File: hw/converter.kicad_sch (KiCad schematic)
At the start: 16 parts, among them J301 1935776, J302 1935776, Q301 SW_L, Q302 SW_H

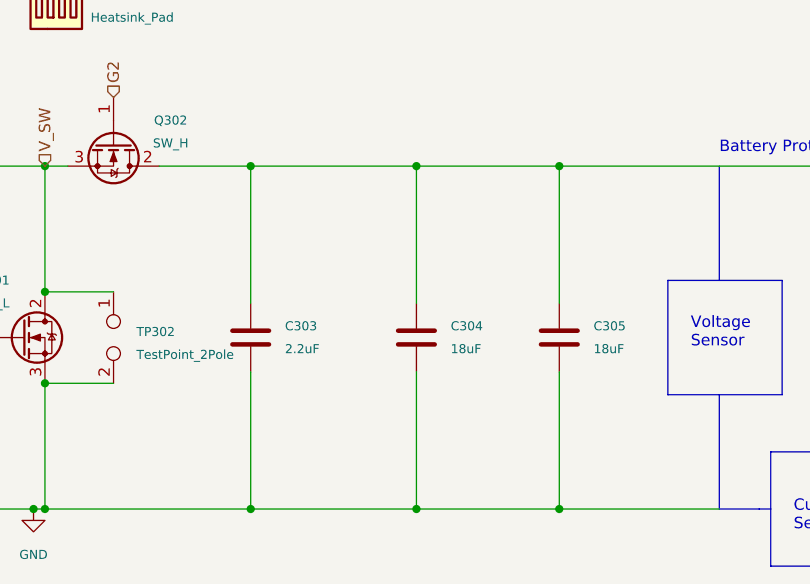
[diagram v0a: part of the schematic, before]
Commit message: hw changes
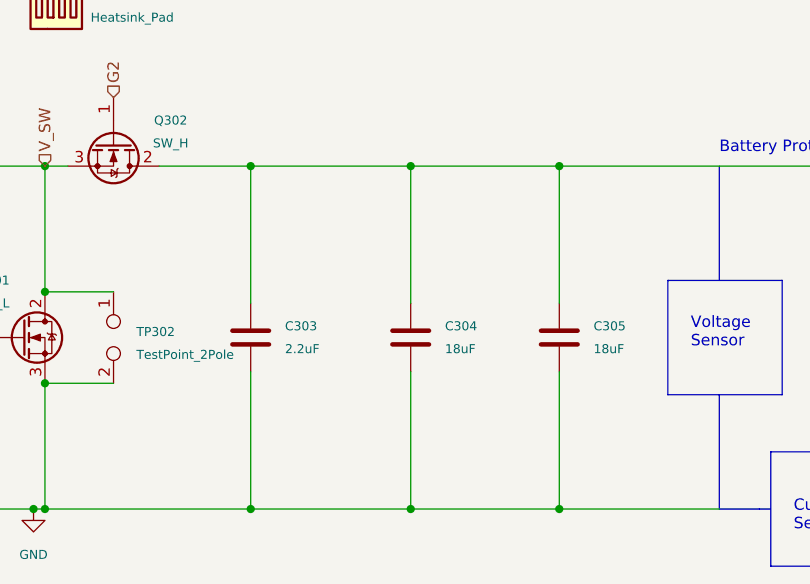
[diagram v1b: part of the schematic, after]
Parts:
- HS301: footprint mppt:WayinTop_HS -> footprints:WayinTop_HS
- J301, J302: footprint mppt:1935776 -> footprints:1935776
- L301: footprint mppt:B65878E1012D001 -> footprints:B65878E1012D001
- Q301, Q302: footprint mppt:EPC2307 -> footprints:EPC2307
- TP302, TP410: footprint mppt:SignalTP -> footprints:SignalTP
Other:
- moved on the sheet: C304
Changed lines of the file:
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@@
   (junction (at 134.62 71.12) (diameter 0) (color 0 0 0 0)
   )
-  (junction (at 198.755 71.12) (diameter 0) (color 0 0 0 0)
+  (junction (at 198.12 71.12) (diameter 0) (color 0 0 0 0)
   )
   (junction (at 157.48 85.09) (diameter 0) (color 0 0 0 0)
@@
   (junction (at 180.34 109.22) (diameter 0) (color 0 0 0 0)
   )
-  (junction (at 198.755 109.22) (diameter 0) (color 0 0 0 0)
+  (junction (at 198.12 109.22) (diameter 0) (color 0 0 0 0)
   )
   (junction (at 156.21 109.22) (diameter 0) (color 0 0 0 0)
@@
     (stroke (width 0) (type default))
   )
-  (wire (pts (xy 180.34 71.12) (xy 198.755 71.12))
+  (wire (pts (xy 180.34 71.12) (xy 198.12 71.12))
     (stroke (width 0) (type default))
   )
@@
     (stroke (width 0) (type default))
   )
-  (wire (pts (xy 198.755 93.98) (xy 198.755 109.22))
+  (wire (pts (xy 198.12 93.98) (xy 198.12 109.22))
     (stroke (width 0) (type default))
   )
@@
     (stroke (width 0) (type default))
   )
-  (wire (pts (xy 198.755 71.12) (xy 214.63 71.12))
+  (wire (pts (xy 198.12 71.12) (xy 214.63 71.12))
     (stroke (width 0) (type default))
   )
@@
     (stroke (width 0) (type default))
   )
-  (wire (pts (xy 180.34 109.22) (xy 198.755 109.22))
+  (wire (pts (xy 180.34 109.22) (xy 198.12 109.22))
     (stroke (width 0) (type default))
   )
@@
     (stroke (width 0) (type default))
   )
-  (wire (pts (xy 198.755 71.12) (xy 198.755 86.36))
+  (wire (pts (xy 198.12 71.12) (xy 198.12 86.36))
     (stroke (width 0) (type default))
   )
@@
     (stroke (width 0) (type default))
   )
-  (wire (pts (xy 198.755 109.22) (xy 214.63 109.22))
+  (wire (pts (xy 198.12 109.22) (xy 214.63 109.22))
     (stroke (width 0) (type default))
   )
@@
       (effects (font (size 1 1)))
     )
-    (property "Footprint" "mppt:1935776" (at 40.64 88.9 0)
+    (property "Footprint" "footprints:1935776" (at 40.64 88.9 0)
       (effects (font (size 1.27 1.27)) (justify bottom) hide)
     )
@@
       (effects (font (size 1 1)) (justify left))
     )
-    (property "Footprint" "mppt:EPC2307" (at 160.02 87.63 0)
+    (property "Footprint" "footprints:EPC2307" (at 160.02 87.63 0)
       (effects (font (size 1.27 1.27)) hide)
     )
@@
       (effects (font (size 1 1)))
     )
-    (property "Footprint" "mppt:1935776" (at 256.54 88.9 0)
+    (property "Footprint" "footprints:1935776" (at 256.54 88.9 0)
       (effects (font (size 1.27 1.27)) (justify bottom) hide)
     )
@@
       (effects (font (size 1 1)))
     )
-    (property "Footprint" "mppt:EPC2307" (at 167.64 73.66 0)
+    (property "Footprint" "footprints:EPC2307" (at 167.64 73.66 0)
       (effects (font (size 1.27 1.27)) hide)
     )
@@
       (effects (font (size 1 1)) (justify left))
     )
-    (property "Footprint" "mppt:SignalTP" (at 114.3 97.79 0)
+    (property "Footprint" "footprints:SignalTP" (at 114.3 97.79 0)
       (effects (font (size 1.27 1.27)) hide)
     )
@@
       (effects (font (size 1 1)) (justify left))
     )
-    (property "Footprint" "mppt:SignalTP" (at 165.1 90.17 0)
+    (property "Footprint" "footprints:SignalTP" (at 165.1 90.17 0)
       (effects (font (size 1.27 1.27)) hide)
     )
@@
       (effects (font (size 1 1)) (justify left))
     )
-    (property "Footprint" "mppt:WayinTop_HS" (at 159.0548 55.88 0)
+    (property "Footprint" "footprints:WayinTop_HS" (at 159.0548 55.88 0)
       (effects (font (size 1.27 1.27)) hide)
     )
@@
     )
   )
-  (symbol (lib_id "Device:C") (at 198.755 90.17 0) (unit 1)
-    (in_bom yes) (on_board yes) (dnp no)
-    (property "Reference" "C304" (at 202.565 88.8999 0)
-      (effects (font (size 1 1)) (justify left))
-    )
-    (property "Value" "18uF" (at 202.565 91.4399 0)
-      (effects (font (size 1 1)) (justify left))
-    )
-    (property "Footprint" "Capacitor_THT:C_Radial_D10.0mm_H16.0mm_P5.00mm" (at 199.7202 93.98 0)
-      (effects (font (size 1.27 1.27)) hide)
-    )
-    (property "Datasheet" "https://www.mouser.com/datasheet/2/212/KEM_A4072_A759-1104329.pdf" (at 198.755 90.17 0)
-      (effects (font (size 1.27 1.27)) hide)
-    )
-    (property "Distributor" "Mouser" (at 198.755 90.17 0)
-      (effects (font (size 1.27 1.27)) hide)
-    )
-    (property "Manufacturer" "KEMET" (at 198.755 90.17 0)
-      (effects (font (size 1.27 1.27)) hide)
-    )
-    (property "P/N" "80-A759MS186M2CAAE90" (at 198.755 90.17 0)
-      (effects (font (size 1.27 1.27)) hide)
-    )
-    (property "LCSC Part #" "" (at 198.755 90.17 0)
-      (effects (font (size 1.27 1.27)) hide)
-    )
-    (property "Cost" "2.58" (at 198.755 90.17 0)
+  (symbol (lib_id "Device:C") (at 198.12 90.17 0) (unit 1)
+    (in_bom yes) (on_board yes) (dnp no)
+    (property "Reference" "C304" (at 201.93 88.8999 0)
+      (effects (font (size 1 1)) (justify left))
+    )
+    (property "Value" "18uF" (at 201.93 91.4399 0)
+      (effects (font (size 1 1)) (justify left))
+    )
+    (property "Footprint" "Capacitor_THT:C_Radial_D10.0mm_H16.0mm_P5.00mm" (at 199.0852 93.98 0)
+      (effects (font (size 1.27 1.27)) hide)
+    )
+    (property "Datasheet" "https://www.mouser.com/datasheet/2/212/KEM_A4072_A759-1104329.pdf" (at 198.12 90.17 0)
+      (effects (font (size 1.27 1.27)) hide)
+    )
+    (property "Distributor" "Mouser" (at 198.12 90.17 0)
+      (effects (font (size 1.27 1.27)) hide)
+    )
+    (property "Manufacturer" "KEMET" (at 198.12 90.17 0)
+      (effects (font (size 1.27 1.27)) hide)
+    )
+    (property "P/N" "80-A759MS186M2CAAE90" (at 198.12 90.17 0)
+      (effects (font (size 1.27 1.27)) hide)
+    )
+    (property "LCSC Part #" "" (at 198.12 90.17 0)
+      (effects (font (size 1.27 1.27)) hide)
+    )
+    (property "Cost" "2.58" (at 198.12 90.17 0)
       (effects (font (size 1.27 1.27)) hide)
     )
@@
       (effects (font (size 1 1)))
     )
-    (property "Footprint" "mppt:B65878E1012D001" (at 101.6 50.8 0)
+    (property "Footprint" "footprints:B65878E1012D001" (at 101.6 50.8 0)
       (effects (font (size 1.27 1.27)) (justify left) hide)
     )
